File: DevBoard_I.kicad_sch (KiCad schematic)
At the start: 9 parts, among them J1 Barrel_Jack_Switch_Pin3Ring, U1 NCP1117-3.3_SOT223, U2 Arduino_UNO_R3, U3 AT25SF081-SSHD-X, U4 AT25SF081-SSHD-X, U5 MCP3550-60-ESN

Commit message: Rev_A Update
U5 footprint change.
Moved J1 and RV1 to the bottom.
Re-route accordingly.
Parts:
- U5: footprint Package_SO:SOIC-8_3.9x4.9mm_P1.27mm -> Package_SO:MSOP-8_3x3mm_P0.65mm
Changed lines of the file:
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@@
       (effects (font (size 1.27 1.27)) (justify left))
     )
-    (property "Footprint" "Package_SO:SOIC-8_3.9x4.9mm_P1.27mm" (id 2) (at 257.81 96.52 0)
+    (property "Footprint" "Package_SO:MSOP-8_3x3mm_P0.65mm" (id 2) (at 257.81 96.52 0)
       (effects (font (size 1.27 1.27) italic) hide)
     )
@@
     )
     (path "/36932855-3ca7-4c22-932c-7ada6196f22c"
-      (reference "U5") (unit 1) (value "MCP3550-60-ESN") (footprint "Package_SO:SOIC-8_3.9x4.9mm_P1.27mm")
-    )
-  )
+      (reference "U5") (unit 1) (value "MCP3550-60-ESN") (footprint "Package_SO:MSOP-8_3x3mm_P0.65mm")
+    )
+  )

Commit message: Added MCP3350 datasheet
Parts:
- U5: footprint Package_SO:MSOP-8_3x3mm_P0.65mm -> Package_SO:SOIC-8_3.9x4.9mm_P1.27mm
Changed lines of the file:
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@@
       (effects (font (size 1.27 1.27)) (justify left))
     )
-    (property "Footprint" "Package_SO:MSOP-8_3x3mm_P0.65mm" (id 2) (at 257.81 96.52 0)
+    (property "Footprint" "Package_SO:SOIC-8_3.9x4.9mm_P1.27mm" (id 2) (at 257.81 96.52 0)
       (effects (font (size 1.27 1.27) italic) hide)
     )
-    (property "Datasheet" "http://ww1.microchip.com/downloads/en/devicedoc/21950c.pdf" (id 3) (at 257.81 96.52 0)
+    (property "Datasheet" "https://ww1.microchip.com/downloads/aemDocuments/documents/OTH/ProductDocuments/DataSheets/20001950F.pdf" (id 3) (at 257.81 96.52 0)
       (effects (font (size 1.27 1.27)) hide)
     )
@@
     )
     (path "/36932855-3ca7-4c22-932c-7ada6196f22c"
-      (reference "U5") (unit 1) (value "MCP3550-60-ESN") (footprint "Package_SO:MSOP-8_3x3mm_P0.65mm")
-    )
-  )
+      (reference "U5") (unit 1) (value "MCP3550-60-ESN") (footprint "Package_SO:SOIC-8_3.9x4.9mm_P1.27mm")
+    )
+  )

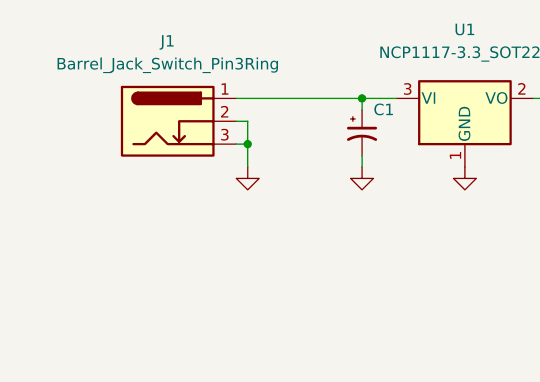
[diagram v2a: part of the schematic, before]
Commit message: N/A
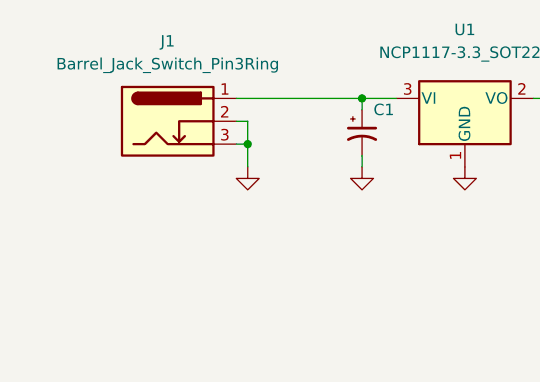
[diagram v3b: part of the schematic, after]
